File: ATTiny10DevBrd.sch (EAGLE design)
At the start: 15 parts, among them IC1 ATTINY10-MAHR

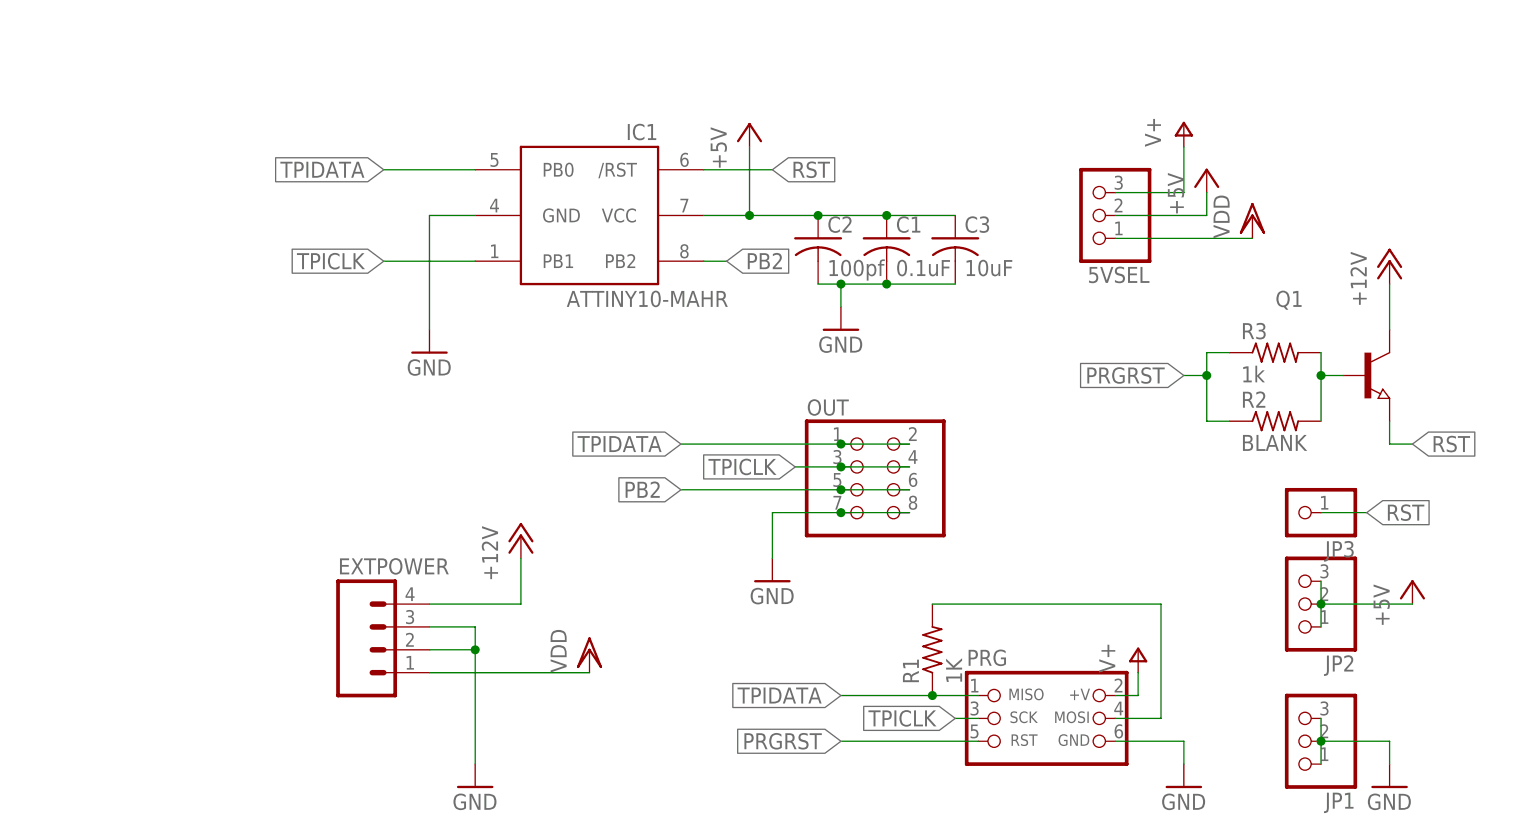
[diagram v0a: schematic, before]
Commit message: Dev board and programmer adapter
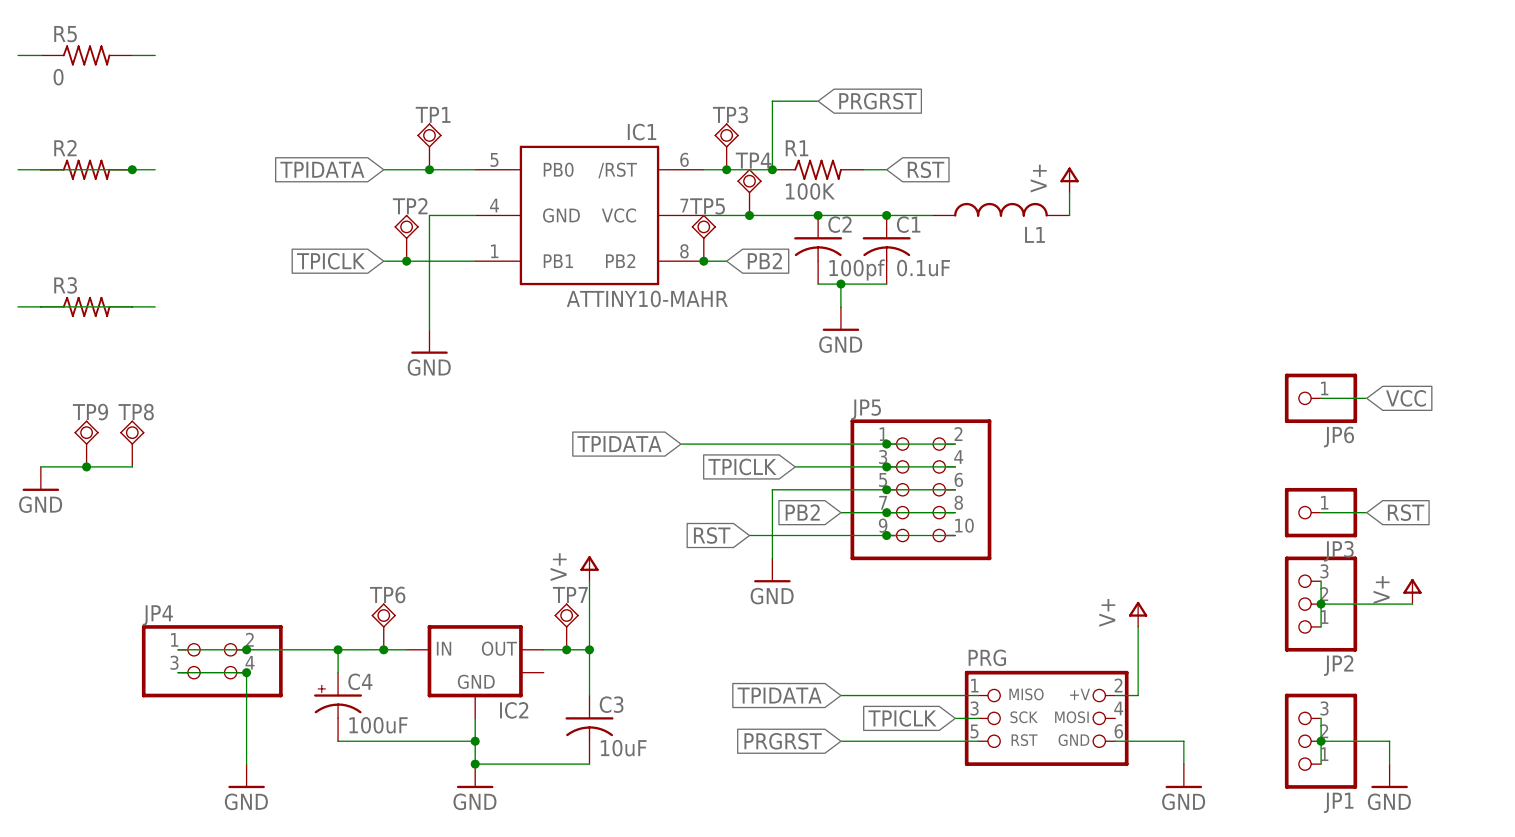
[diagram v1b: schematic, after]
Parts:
- removed 5VSEL: (no value), adafruit:PINHD-1X3CB
- removed EXTPOWER: (no value), LL:HEADER1X4SMD_LONGPADS
- removed OUT: (no value), adafruit:PINHD-2X4
- removed Q1: (no value), semicon-smd-ipc:NPN-TRANSISTOR_SOT23
- added C4: 100uF, LL:CPOL-USE
- added IC2: (no value), LL:V_REG_LM1117SOT223
- added JP4: (no value), pinhead:PINHD-2X2
- added JP5: (no value), pinhead:PINHD-2X5
- added JP6: (no value), adafruit:PINHD-1X1
- added L1: (no value), LL:L-USL1812
- added R5: 0, LL:R-US_M0805
- added TP1, TP2, TP3, TP4, TP5, TP6, TP7, TP8, TP9: TPSQTP12R, testpad:TPSQTP12R
- C3: device adafruit:C-USC0805 -> LL:C-USC0805K
- R1: value 1K -> 100K
- R2: value BLANK -> (none); device adafruit:R-US_R0805 -> LL:R-US_M1206
- R3: value 1k -> (none); device adafruit:R-US_R0805 -> LL:R-US_M1206
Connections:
- removed net +12V: EXTPOWER.4, Q1.C
- removed net +5V: 5VSEL.2, C1.1, C2.1, C3.1, IC1.VCC, JP2.1, JP2.2, JP2.3
- removed net N$1: Q1.B, R2.2, R3.2
- removed net N$5: PRG.MOSI, R1.2
- removed net VDD: 5VSEL.1, EXTPOWER.1
- new net VCC: C1.1, C2.1, IC1.VCC, JP6.1, L1.1, TP4.TP
- new net VIN: C4.+, IC2.IN, JP4.1, JP4.2, TP6.TP
- net GND: now also C4.-, IC2.GND, JP4.3, JP4.4, JP5.5, JP5.6, TP8.TP, TP9.TP; no longer EXTPOWER.2, EXTPOWER.3, OUT.7, OUT.8
- net PB2: now also JP5.7, JP5.8, R3.1, R3.2, TP5.TP; no longer OUT.5, OUT.6
- net PRGRST: now also IC1./RST, R1.1, TP3.TP; no longer R2.1, R3.1
- net RST: now also JP5.10, JP5.9, R1.2; no longer IC1./RST, Q1.E
- net TPICLK: now also JP5.3, JP5.4, R2.1, R2.2, TP2.TP; no longer OUT.3, OUT.4
- net TPIDATA: now also JP5.1, JP5.2, R5.1, R5.2, TP1.TP; no longer OUT.1, OUT.2, R1.1
- net V+: now also C3.1, IC2.VR-OUTSM, JP2.1, JP2.2, JP2.3, L1.2, TP7.TP; no longer 5VSEL.3
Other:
- moved on the sheet: C3, R1, R2, R3
